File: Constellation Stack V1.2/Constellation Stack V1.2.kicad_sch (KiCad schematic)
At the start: 95 parts, among them J1 PWR_IN, J2 USB_C_Receptacle_USB2.0, J3 RS485 Out, J4 PT_IN, J5 GPIO_OUT, J6 CAN_TERMINAL, Q1 MBT2222ADW1T1, SW1 RESET, SW2 SW_SPST, SW3 GPIO_0, U1 ESP32-PICO-MINI-02, U2 TJA1050T_CM_118, U3 CP2102N-Axx-xQFN24, U4 AP62150Z6-7, U5 TCR2EF50_LMCT, U6 TLV1117LV33DCYR, U7 ADS8684, U8 MAX485CSA+T, U9 W25Q16JVSSIQ

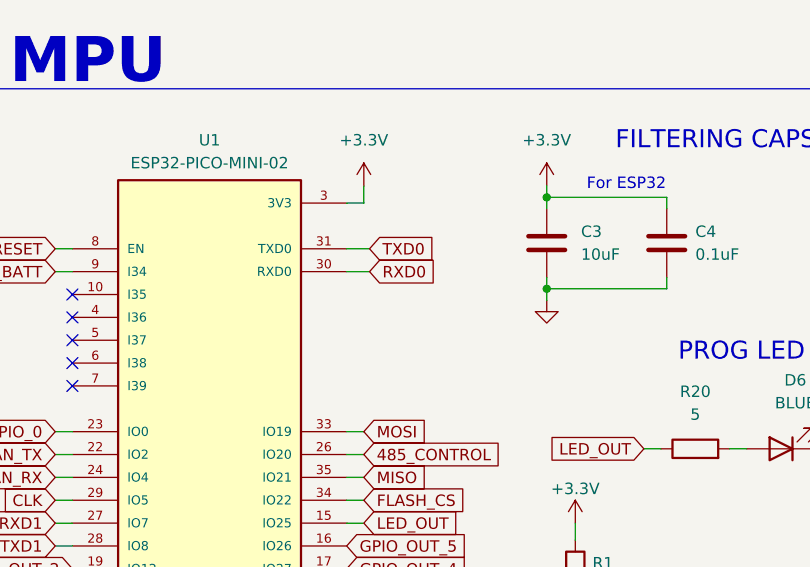
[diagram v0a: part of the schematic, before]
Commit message: Ahhhahahaha
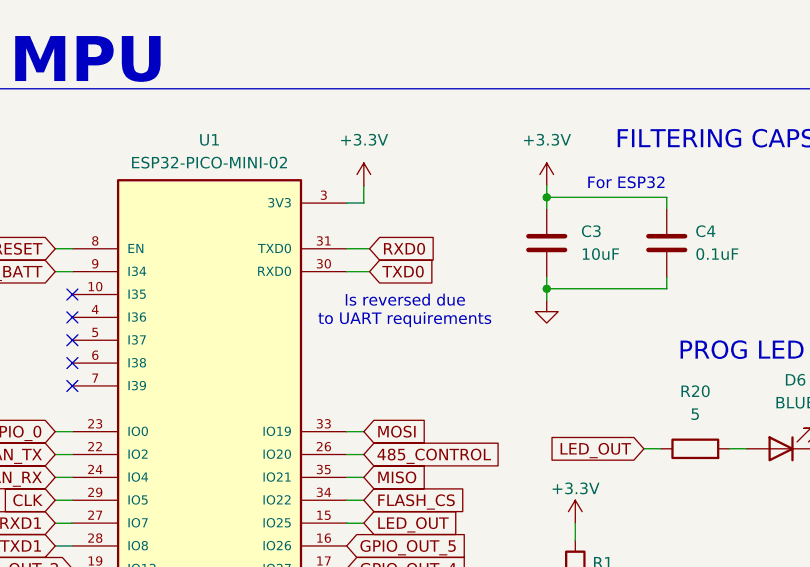
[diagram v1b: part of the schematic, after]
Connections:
- net RXD0: now also U1.31 (TXD0); no longer U1.30 (RXD0)
- net TXD0: now also U1.30 (RXD0); no longer U1.31 (TXD0)
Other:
- note added: "Is reversed due to UART requirements"
